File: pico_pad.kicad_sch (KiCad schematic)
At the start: 26 parts, among them J1 Conn_01x20_Pin, J2 Conn_01x20_Pin, J3 Conn_01x10_Pin, J4 Conn_01x10_Pin, SW1 SW_Push, SW10 SW_Push, SW11 SW_Push, SW2 SW_Push, SW3 SW_Push, SW4 SW_Push, SW5 SW_Push, SW6 SW_Push, SW7 SW_Push, SW8 SW_Push, SW9 SW_Push

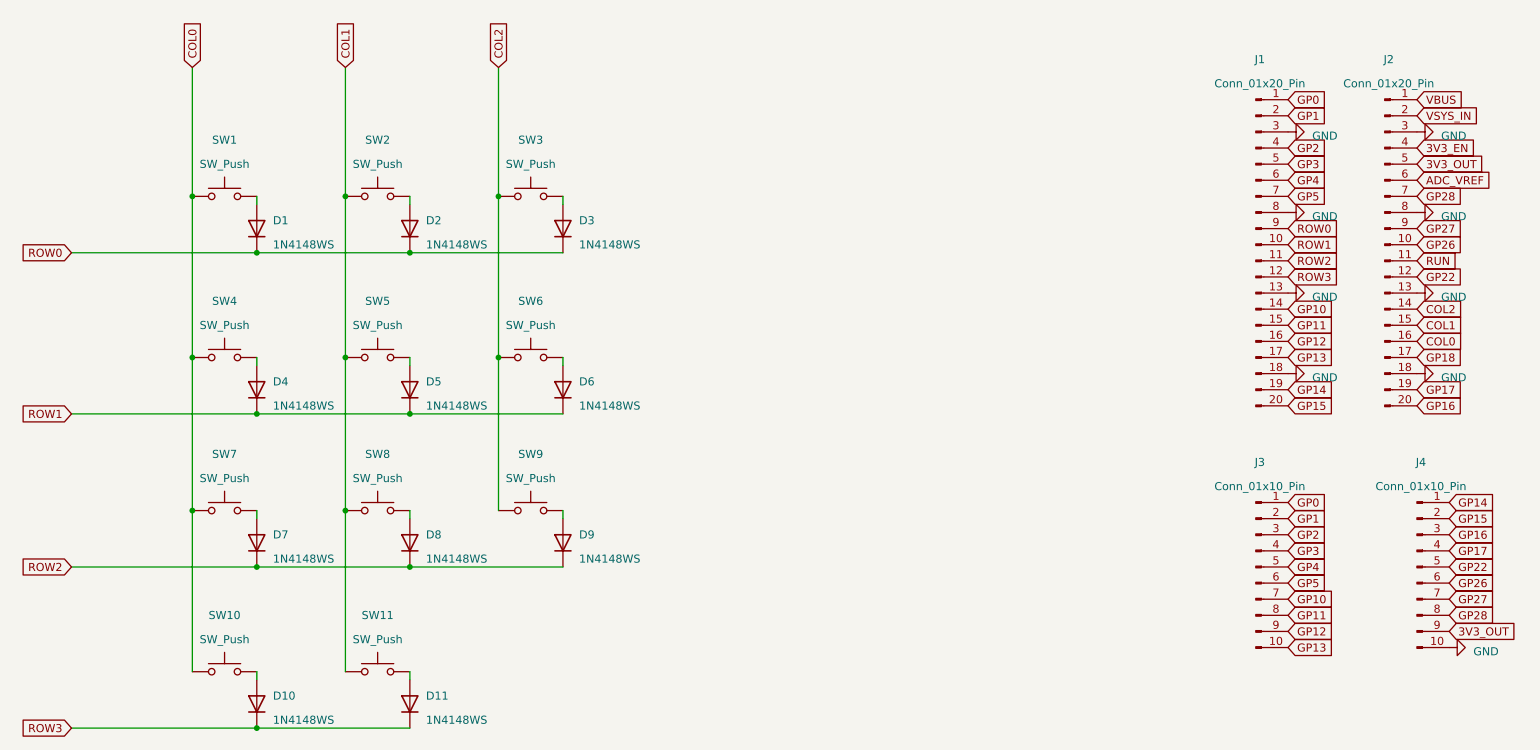
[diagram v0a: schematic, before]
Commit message: update pcb
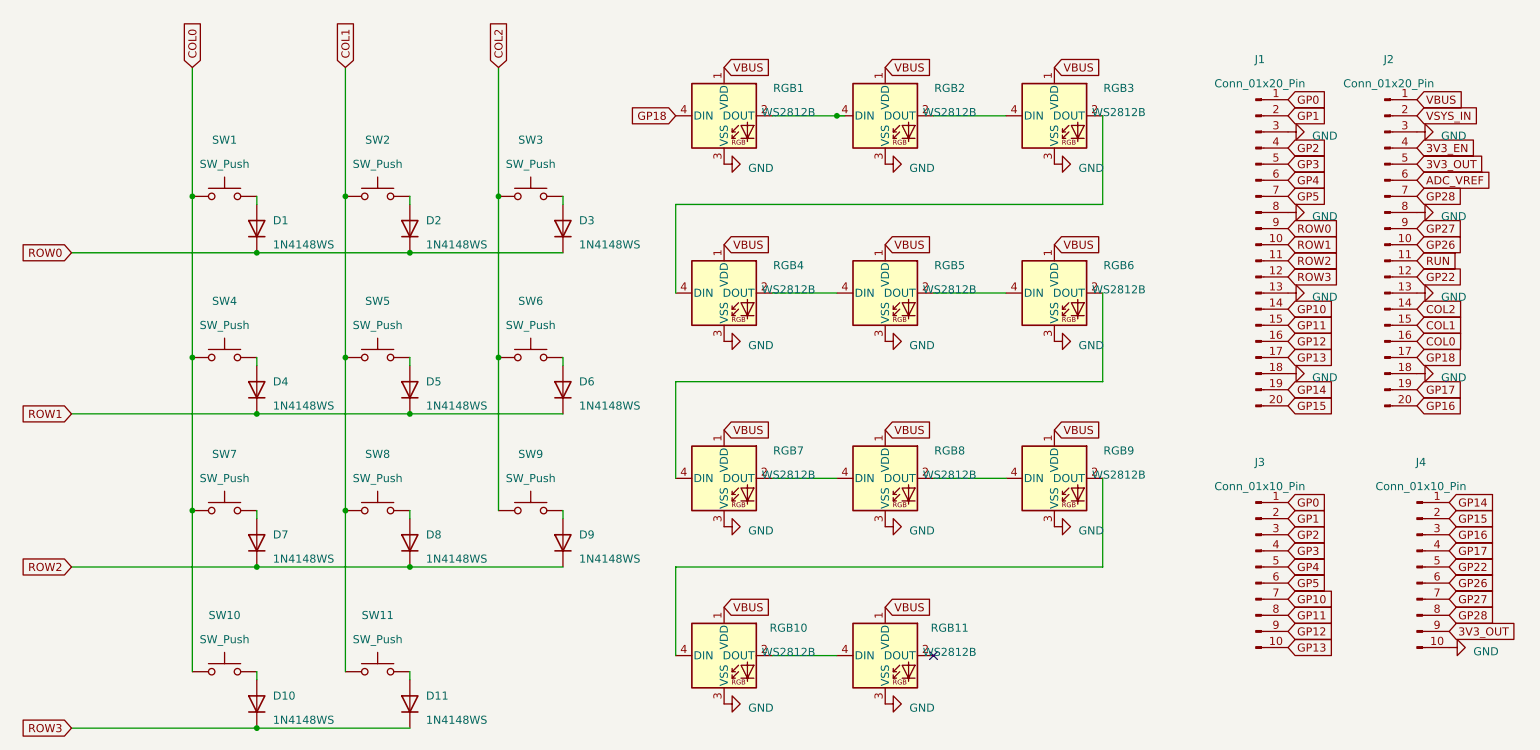
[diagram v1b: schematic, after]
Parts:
- added RGB1, RGB10, RGB11, RGB2, RGB3, RGB4, RGB5, RGB6, RGB7, RGB8, RGB9: WS2812B, LED_SMD:LED_WS2812B-2020_PLCC4_2.0x2.0mm, symbol LED:WS2812B
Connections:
- net GND: now also RGB1.3 (VSS), RGB10.3 (VSS), RGB11.3 (VSS), RGB2.3 (VSS), RGB3.3 (VSS), RGB4.3 (VSS), RGB5.3 (VSS), RGB6.3 (VSS), RGB7.3 (VSS), RGB8.3 (VSS), RGB9.3 (VSS)
- net GP18: now also RGB1.4 (DIN)
- net VBUS: now also RGB1.1 (VDD), RGB10.1 (VDD), RGB11.1 (VDD), RGB2.1 (VDD), RGB3.1 (VDD), RGB4.1 (VDD), RGB5.1 (VDD), RGB6.1 (VDD), RGB7.1 (VDD), RGB8.1 (VDD), RGB9.1 (VDD)
- new net: RGB7.2 (DOUT), RGB8.4 (DIN)
- new net: RGB6.2 (DOUT), RGB7.4 (DIN)
- new net: RGB4.2 (DOUT), RGB5.4 (DIN)
- new net: RGB3.2 (DOUT), RGB4.4 (DIN)
- new net: RGB10.2 (DOUT), RGB11.4 (DIN)
- new net: RGB1.2 (DOUT), RGB2.4 (DIN)
- new net: RGB8.2 (DOUT), RGB9.4 (DIN)
- new net: RGB2.2 (DOUT), RGB3.4 (DIN)
- new net: RGB5.2 (DOUT), RGB6.4 (DIN)
- new net: RGB10.4 (DIN), RGB9.2 (DOUT)
- no-connect marks 0 -> 1

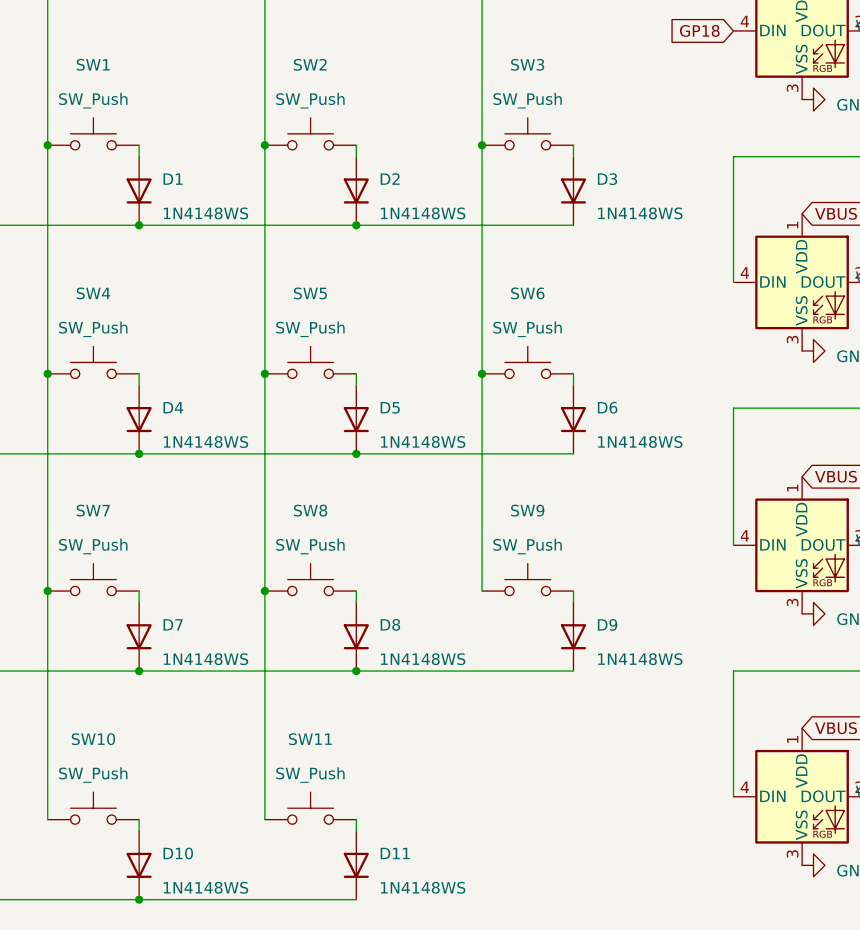
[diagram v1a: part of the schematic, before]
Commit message: update
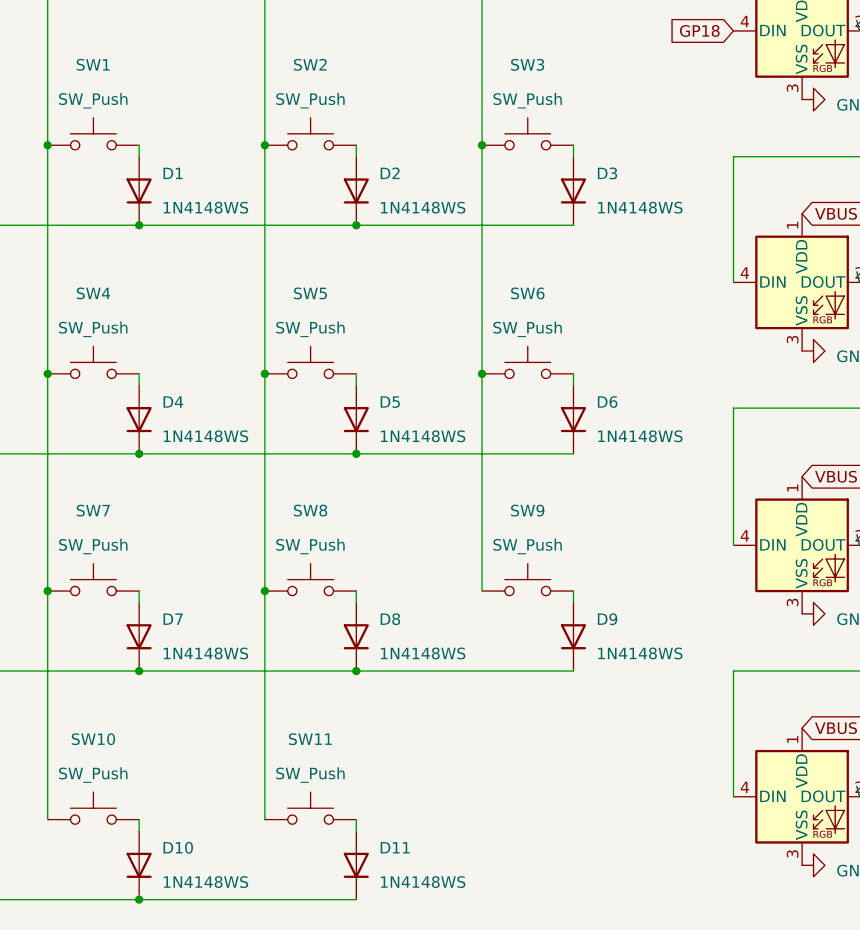
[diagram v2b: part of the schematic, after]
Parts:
- D1, D10, D11, D2, D3, D4, D5, D6, D7, D8, D9: footprint Diode_SMD:D_SOD-323 -> Diode_SMD:D_SOD-123; symbol Diode:1N4148WS -> Diode:1N4148W

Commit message: update pcb, add ws2812
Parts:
- RGB1, RGB10, RGB11, RGB2, RGB3, RGB4, RGB5, RGB6, RGB7, RGB8, RGB9: footprint LED_SMD:LED_WS2812B-2020_PLCC4_2.0x2.0mm -> LED_SMD:LED-SMD_L3.2-W2.8-BR_DY-S352818
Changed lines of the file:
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@@
       (effects (font (size 1.27 1.27)))
     )
-    (property "Footprint" "LED_SMD:LED_WS2812B-2020_PLCC4_2.0x2.0mm" (at 130.81 97.79 0)
+    (property "Footprint" "LED_SMD:LED-SMD_L3.2-W2.8-BR_DY-S352818" (at 130.81 97.79 0)
       (effects (font (size 1.27 1.27)) (justify left top) hide)
     )
@@
       (effects (font (size 1.27 1.27)))
     )
-    (property "Footprint" "LED_SMD:LED_WS2812B-2020_PLCC4_2.0x2.0mm" (at 130.81 68.58 0)
+    (property "Footprint" "LED_SMD:LED-SMD_L3.2-W2.8-BR_DY-S352818" (at 130.81 68.58 0)
       (effects (font (size 1.27 1.27)) (justify left top) hide)
     )
@@
       (effects (font (size 1.27 1.27)))
     )
-    (property "Footprint" "LED_SMD:LED_WS2812B-2020_PLCC4_2.0x2.0mm" (at 156.21 125.73 0)
+    (property "Footprint" "LED_SMD:LED-SMD_L3.2-W2.8-BR_DY-S352818" (at 156.21 125.73 0)
       (effects (font (size 1.27 1.27)) (justify left top) hide)
     )
@@
       (effects (font (size 1.27 1.27)))
     )
-    (property "Footprint" "LED_SMD:LED_WS2812B-2020_PLCC4_2.0x2.0mm" (at 130.81 40.64 0)
+    (property "Footprint" "LED_SMD:LED-SMD_L3.2-W2.8-BR_DY-S352818" (at 130.81 40.64 0)
       (effects (font (size 1.27 1.27)) (justify left top) hide)
     )
@@
       (effects (font (size 1.27 1.27)))
     )
-    (property "Footprint" "LED_SMD:LED_WS2812B-2020_PLCC4_2.0x2.0mm" (at 156.21 97.79 0)
+    (property "Footprint" "LED_SMD:LED-SMD_L3.2-W2.8-BR_DY-S352818" (at 156.21 97.79 0)
       (effects (font (size 1.27 1.27)) (justify left top) hide)
     )
@@
       (effects (font (size 1.27 1.27)))
     )
-    (property "Footprint" "LED_SMD:LED_WS2812B-2020_PLCC4_2.0x2.0mm" (at 156.21 40.64 0)
+    (property "Footprint" "LED_SMD:LED-SMD_L3.2-W2.8-BR_DY-S352818" (at 156.21 40.64 0)
       (effects (font (size 1.27 1.27)) (justify left top) hide)
     )
@@
       (effects (font (size 1.27 1.27)))
     )
-    (property "Footprint" "LED_SMD:LED_WS2812B-2020_PLCC4_2.0x2.0mm" (at 182.88 68.58 0)
+    (property "Footprint" "LED_SMD:LED-SMD_L3.2-W2.8-BR_DY-S352818" (at 182.88 68.58 0)
       (effects (font (size 1.27 1.27)) (justify left top) hide)
     )
@@
       (effects (font (size 1.27 1.27)))
     )
-    (property "Footprint" "LED_SMD:LED_WS2812B-2020_PLCC4_2.0x2.0mm" (at 182.88 97.79 0)
+    (property "Footprint" "LED_SMD:LED-SMD_L3.2-W2.8-BR_DY-S352818" (at 182.88 97.79 0)
       (effects (font (size 1.27 1.27)) (justify left top) hide)
     )
@@
       (effects (font (size 1.27 1.27)))
     )
-    (property "Footprint" "LED_SMD:LED_WS2812B-2020_PLCC4_2.0x2.0mm" (at 182.88 40.64 0)
+    (property "Footprint" "LED_SMD:LED-SMD_L3.2-W2.8-BR_DY-S352818" (at 182.88 40.64 0)
       (effects (font (size 1.27 1.27)) (justify left top) hide)
     )
@@
       (effects (font (size 1.27 1.27)))
     )
-    (property "Footprint" "LED_SMD:LED_WS2812B-2020_PLCC4_2.0x2.0mm" (at 130.81 125.73 0)
+    (property "Footprint" "LED_SMD:LED-SMD_L3.2-W2.8-BR_DY-S352818" (at 130.81 125.73 0)
       (effects (font (size 1.27 1.27)) (justify left top) hide)
     )
@@
       (effects (font (size 1.27 1.27)))
     )
-    (property "Footprint" "LED_SMD:LED_WS2812B-2020_PLCC4_2.0x2.0mm" (at 156.21 68.58 0)
-      (effects (font (size 1.27 1.27)) (justify left top) hide)
-    )
+    (property "Footprint" "LED_SMD:LED-SMD_L3.2-W2.8-BR_DY-S352818" (at 156.21 68.58 0)
+      (effects (font (size 1.27 1.27)) (justify left top) hide)
+    )
